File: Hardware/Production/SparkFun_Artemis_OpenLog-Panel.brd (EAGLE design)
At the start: 106.2 x 95.2 mm, 714 parts, among them J11 QWIIC_RIGHT_ANGLE, J14 CORTEX_JTAG, J16 CORTEX_JTAG, J17 MICRO-SD, J18 MICRO-SD, J19 QWIIC_RIGHT_ANGLE, J25 CORTEX_JTAG, J26 MICRO-SD, J27 QWIIC_RIGHT_ANGLE, J33 CORTEX_JTAG, J34 MICRO-SD, J35 QWIIC_RIGHT_ANGLE, J41 CORTEX_JTAG, J42 MICRO-SD, J43 QWIIC_RIGHT_ANGLE, J6 CORTEX_JTAG, J7 MICRO-SD, J8 QWIIC_RIGHT_ANGLE, Q1 20V/0.2A/8MHz/1.2Ω/1Vth, Q10 20V/0.2A/8MHz/1.2Ω/1Vth, Q11 20V/0.2A/8MHz/1.2Ω/1Vth, Q12 20V/4.2A/52mΩ/1.4W, Q13 20V/0.2A/8MHz/1.2Ω/1Vth, Q14 20V/0.2A/8MHz/1.2Ω/1Vth, Q15 20V/0.2A/8MHz/1.2Ω/1Vth, Q16 20V/0.2A/8MHz/1.2Ω/1Vth, Q17 20V/0.2A/8MHz/1.2Ω/1Vth, Q18 20V/4.2A/52mΩ/1.4W, Q19 20V/0.2A/8MHz/1.2Ω/1Vth, Q2 20V/0.2A/8MHz/1.2Ω/1Vth, Q20 20V/0.2A/8MHz/1.2Ω/1Vth, Q21 20V/0.2A/8MHz/1.2Ω/1Vth, Q22 20V/0.2A/8MHz/1.2Ω/1Vth, Q23 20V/0.2A/8MHz/1.2Ω/1Vth, Q24 20V/4.2A/52mΩ/1.4W, Q25 20V/0.2A/8MHz/1.2Ω/1Vth, Q26 20V/0.2A/8MHz/1.2Ω/1Vth, Q27 20V/0.2A/8MHz/1.2Ω/1Vth, Q28 20V/0.2A/8MHz/1.2Ω/1Vth, Q29 20V/0.2A/8MHz/1.2Ω/1Vth, Q3 20V/0.2A/8MHz/1.2Ω/1Vth, Q30 20V/4.2A/52mΩ/1.4W, Q31 20V/0.2A/8MHz/1.2Ω/1Vth, Q32 20V/0.2A/8MHz/1.2Ω/1Vth, Q33 20V/0.2A/8MHz/1.2Ω/1Vth, Q34 20V/0.2A/8MHz/1.2Ω/1Vth, Q35 20V/0.2A/8MHz/1.2Ω/1Vth, Q36 20V/4.2A/52mΩ/1.4W, Q4 20V/4.2A/52mΩ/1.4W, Q5 20V/0.2A/8MHz/1.2Ω/1Vth, Q6 20V/0.2A/8MHz/1.2Ω/1Vth, Q7 20V/0.2A/8MHz/1.2Ω/1Vth, Q8 20V/0.2A/8MHz/1.2Ω/1Vth, Q9 20V/0.2A/8MHz/1.2Ω/1Vth, U1 3.2V Supervisor, U10 CH340E, U11 AP2112K, U12 3.2V Supervisor, U13 ICM-20948, U14 1.8V/100mA, U15 MCP73831, U16 ARTEMIS_MODULESMD, U17 CH340E, U18 ICM-20948, U19 1.8V/100mA, U2 MCP73831, U20 AP2112K, U21 3.2V Supervisor, U22 MCP73831, U23 ARTEMIS_MODULESMD, U24 CH340E, U25 ICM-20948, U26 1.8V/100mA, U27 AP2112K, U28 3.2V Supervisor, U29 MCP73831, U3 AP2112K, U30 ARTEMIS_MODULESMD, U31 CH340E, U32 ICM-20948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

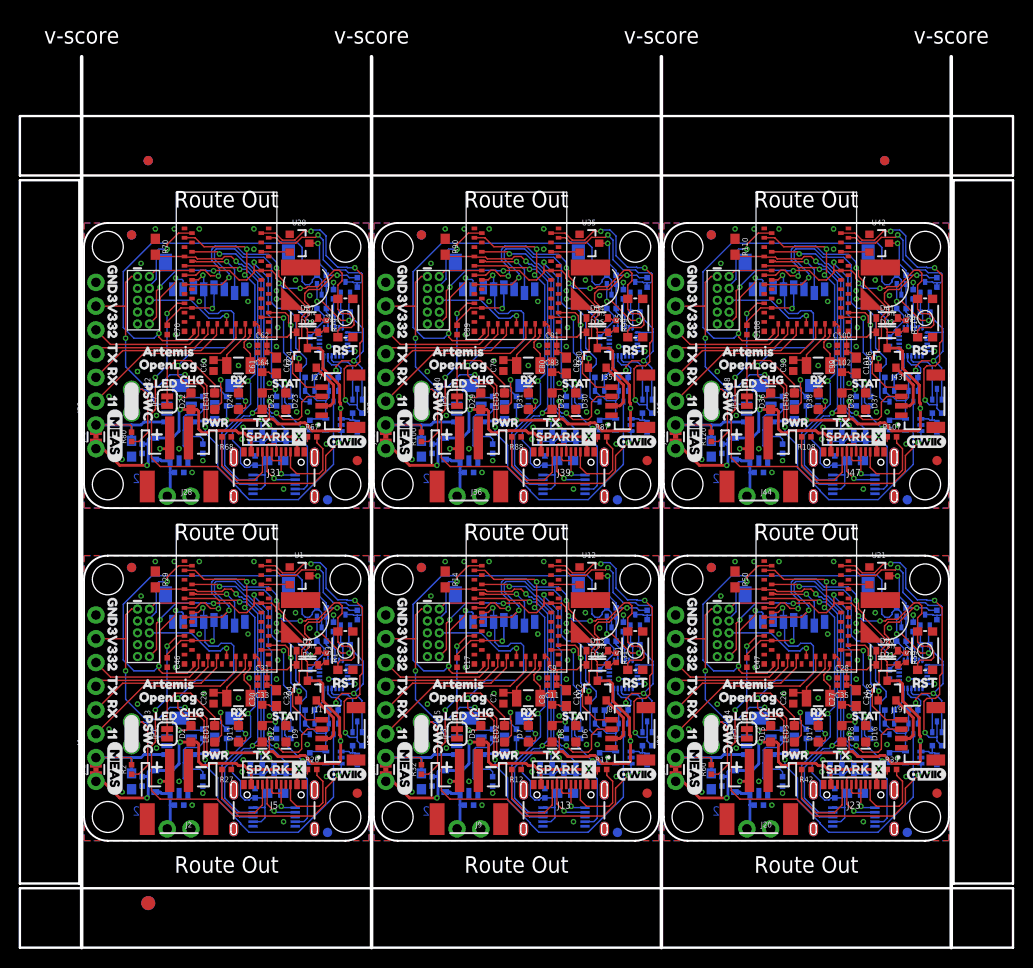
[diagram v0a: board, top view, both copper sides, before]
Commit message: PCB x03 commit for fab.
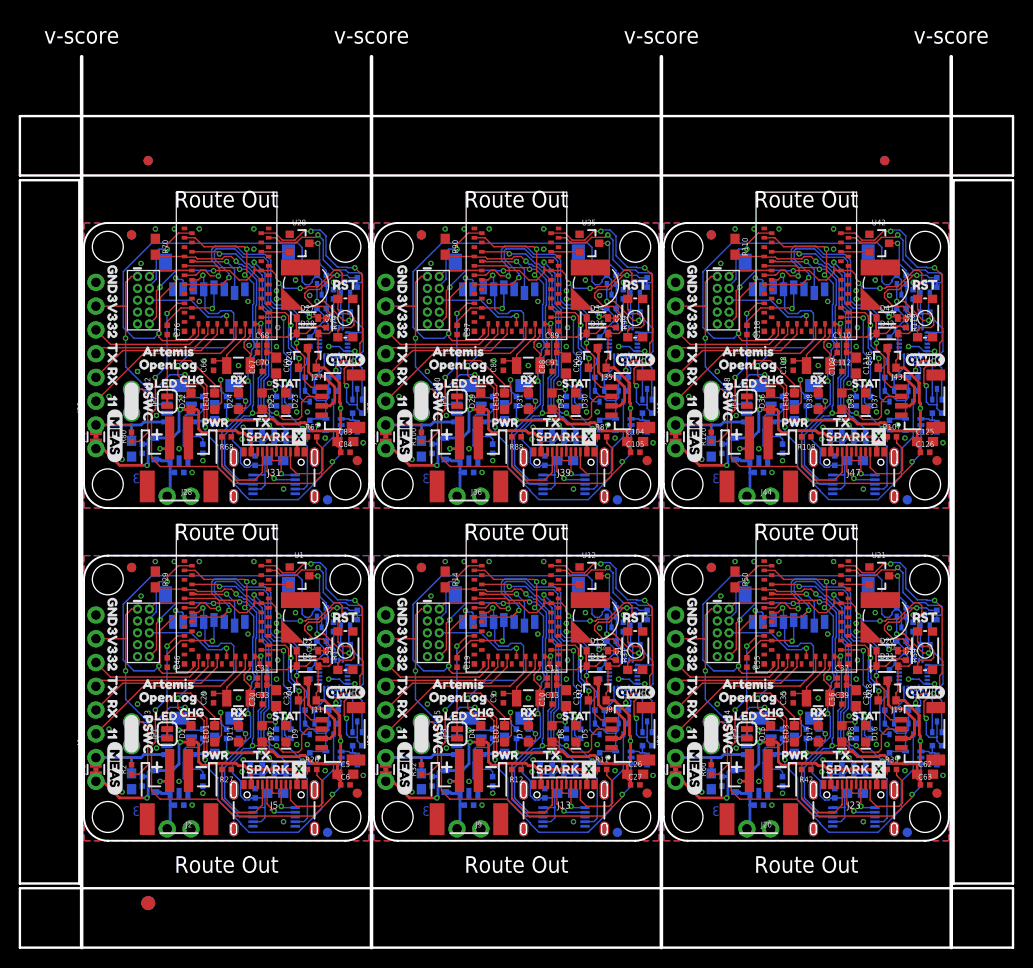
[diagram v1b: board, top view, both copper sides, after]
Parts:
- added C115, C116, C118, C119, C120: 0.1uF, SparkFun-Capacitors:0402-TIGHT
- added C117: 1.0nF, SparkFun-Capacitors:0402-TIGHT
- added C121, C122, C126: 1.0uF, SparkFun-Capacitors:0402-TIGHT
- added C123: 1.0uF, SparkFun-Capacitors:0603
- added C124: 2.2uF, SparkFun-Capacitors:0603
- added C125: 10uF, SparkFun-Capacitors:0603
- BT1, BT2, BT3, BT4, BT5, BT6: value ML414H_IV01E_BATTERY -> ML414H
- C10: value 10uF -> 15pF; device SparkFun-Capacitors:0603 -> SparkFun-Capacitors:0402-TIGHT
- C100, C105, C13, C39, C70, C91: value 0.1uF -> 1.0uF
- C101, C63: value 10uF -> 1.0uF; device SparkFun-Capacitors:0603 -> SparkFun-Capacitors:0402-TIGHT
- C102: device SparkFun-Capacitors:0402-TIGHT -> SparkFun-Capacitors:0603
- C103: value 10nF -> 2.2uF
- C104, C38, C62, C90: value 0.1uF -> 10uF; device SparkFun-Capacitors:0402-TIGHT -> SparkFun-Capacitors:0603
- C106, C28, C85, C86: value 0.1uF -> 4.7uF
- C107: value 1.0nF -> 4.7uF
- C108, C109, C66, C67, C87, C9: value 0.1uF -> 15pF
- C11, C20, C21, C55, C73, C74, C93: value 1.0uF -> 0.1uF
- C111, C83: value 1.0uF -> 10uF; device SparkFun-Capacitors:0402-TIGHT -> SparkFun-Capacitors:0603
- C113: value 1.0uF -> 10nF
- C114, C57, C76, C95: value 2.2uF -> 0.1uF; device SparkFun-Capacitors:0603 -> SparkFun-Capacitors:0402-TIGHT
- C12: value 10nF -> 10uF
- C14, C71: value 0.1uF -> 10nF; device SparkFun-Capacitors:0402-TIGHT -> SparkFun-Capacitors:0603
- C16: value 1.0nF -> 0.1uF
- C18: value 0.1uF -> 1.0nF
- C22: device SparkFun-Capacitors:0603 -> SparkFun-Capacitors:0402-TIGHT
- C23: value 2.2uF -> 1.0uF; device SparkFun-Capacitors:0603 -> SparkFun-Capacitors:0402-TIGHT
- C24: value 4.7uF -> 1.0uF; device SparkFun-Capacitors:0402-TIGHT -> SparkFun-Capacitors:0603
- C25: value 4.7uF -> 2.2uF; device SparkFun-Capacitors:0402-TIGHT -> SparkFun-Capacitors:0603
- C26: value 15pF -> 10uF; device SparkFun-Capacitors:0402 -> SparkFun-Capacitors:0603
- C27, C79, C80: value 15pF -> 1.0uF; device SparkFun-Capacitors:0402 -> SparkFun-Capacitors:0402-TIGHT
- C29, C30: device SparkFun-Capacitors:0402 -> SparkFun-Capacitors:0402-TIGHT
- C34: value 10uF -> 4.7uF; device SparkFun-Capacitors:0603 -> SparkFun-Capacitors:0402-TIGHT
- C35: value 1.0uF -> 15pF
- C36: value 10nF -> 15pF; device SparkFun-Capacitors:0603 -> SparkFun-Capacitors:0402-TIGHT
- C45: value 1.0nF -> 10nF; device SparkFun-Capacitors:0402-TIGHT -> SparkFun-Capacitors:0603
- C5: value 4.7uF -> 10uF; device SparkFun-Capacitors:0402-TIGHT -> SparkFun-Capacitors:0603
- C50: value 1.0uF -> 1.0nF
- C56, C94: value 1.0uF -> 0.1uF; device SparkFun-Capacitors:0603 -> SparkFun-Capacitors:0402-TIGHT
- C58, C59, C6: value 4.7uF -> 1.0uF
- C60: value 15pF -> 1.0uF; device SparkFun-Capacitors:0402 -> SparkFun-Capacitors:0603
- C61: value 15pF -> 2.2uF; device SparkFun-Capacitors:0402 -> SparkFun-Capacitors:0603
- C64: value 1.0uF -> 4.7uF
- C65: value 10nF -> 4.7uF; device SparkFun-Capacitors:0603 -> SparkFun-Capacitors:0402-TIGHT
- C69: value 1.0nF -> 10uF; device SparkFun-Capacitors:0402-TIGHT -> SparkFun-Capacitors:0603
- C7, C8: value 15pF -> 4.7uF; device SparkFun-Capacitors:0402 -> SparkFun-Capacitors:0402-TIGHT
- C75: value 1.0uF -> 1.0nF; device SparkFun-Capacitors:0603 -> SparkFun-Capacitors:0402-TIGHT
- C77, C78, C97: value 4.7uF -> 0.1uF
- C81: value 0.1uF -> 1.0uF; device SparkFun-Capacitors:0402-TIGHT -> SparkFun-Capacitors:0603
- C82: value 10uF -> 2.2uF
- C84: value 10nF -> 1.0uF; device SparkFun-Capacitors:0603 -> SparkFun-Capacitors:0402-TIGHT
- C88: value 1.0nF -> 15pF
- C92: value 1.0uF -> 10nF; device SparkFun-Capacitors:0402-TIGHT -> SparkFun-Capacitors:0603
- C96: value 4.7uF -> 1.0nF
- C98, C99: value 15pF -> 0.1uF; device SparkFun-Capacitors:0402 -> SparkFun-Capacitors:0402-TIGHT
- D14, D21, D28, D35, D42: value 3A/10V/280mV -> 1A/23V/620mV
- D4: value 3A/10V/280mV -> Yellow; device SparkFun-DiscreteSemi:SOD-323 -> SparkFun-LED:LED-0603
- D5: value Yellow -> BLUE
- D6: value BLUE -> 1A/23V/620mV; device SparkFun-LED:LED-0603 -> SparkFun-DiscreteSemi:SOD-323
- J11, J19, J27, J35, J43, J8: value QWIIC_RIGHT_ANGLE -> (none)
- moved C59 91.2 mm to (91.2, 8.64)
- moved C62 84.4 mm to (89.9, 7.11)
- moved C63 82.6 mm to (89.9, 5.97), turned to 0 degrees
- moved C58 79.0 mm to (86.1, 17.8), turned to 270 degrees
- moved C61 69.8 mm to (75.9, 10.2), flipped to the bottom
- moved C60 69.3 mm to (67.1, 6.35), flipped to the bottom, turned to 270 degrees
- moved C81 46.3 mm to (5.08, 41.9), flipped to the bottom, turned to 270 degrees
- moved C102 46.1 mm to (36.1, 41.9), flipped to the bottom, turned to 270 degrees
- moved C82 37.9 mm to (14.0, 45.7), flipped to the bottom, turned to 90 degrees
- moved C103 37.8 mm to (45.0, 45.7), turned to 90 degrees
- moved C24 36.2 mm to (36.1, 6.35), turned to 270 degrees
- moved C97 31.0 mm to (39.9, 54.6), flipped to the top
- moved D6 29.6 mm to (23.9, 18.7), turned to 0 degrees
- moved C56 27.2 mm to (88.6, 22.9), turned to 90 degrees
- moved C99 26.6 mm to (55.1, 44.5), flipped to the bottom, turned to 270 degrees
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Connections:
- net 3.3V: now also C5.1, C6.1, D6.A, Q4.2; no longer D4.A, Q4.3, R1.2, R28.2
- net 3.3V1: now also C14.1, C15.1, C25.1, C26.1, C27.1, Q12.2; no longer C12.1, C13.1, C21.1, Q12.3, R13.2, R31.2
- net 3.3V2: now also C45.1, C47.1, C59.1, C61.1, C62.1, C63.1, Q18.2; no longer C36.1, C37.1, C55.1, C57.1, Q18.3, R43.2, R59.2
- net 3.3V3: now also C71.1, C72.1, C80.1, C82.1, C83.1, C84.1, Q24.2; no longer C65.1, C66.1, C74.1, C76.1, Q24.3, R69.2, R79.2
- net 3.3V4: now also C101.1, C103.1, C104.1, C105.1, C92.1, Q30.2; no longer C84.1, C85.1, C95.1, Q30.3, R89.2, R99.2
- net 3.3V5: now also C113.1, C122.1, C124.1, C125.1, C126.1, Q36.2; no longer C103.1, C104.1, C112.1, Q36.3, R109.2, R119.2
- net 5V1: now also C8.1, D4.A; no longer C6.1, D5.A
- net 5V2: now also C34.1; no longer C25.1
- net 5V3: now also C65.1; no longer C59.1
- net 5V4: now also C86.1; no longer C78.1
- net 5V5: now also C107.1; no longer C97.1
- net ARTEMIS_!RESET1: now also C16.2, C18.1; no longer C14.2, C16.1
- net ARTEMIS_!RESET2: now also C48.2, C50.1; no longer C38.2, C45.1
- net ARTEMIS_!RESET3: now also C73.2, C75.1; no longer C67.2, C69.1
- net ARTEMIS_!RESET4: now also C94.2, C96.1; no longer C86.2, C88.1
- net ARTEMIS_!RESET5: now also C115.2, C117.1; no longer C105.2, C107.1
- net ARTEMIS_!RTS!1: now also C16.1, C17.1; no longer C14.1, C15.1
- net ARTEMIS_!RTS!2: now also C48.1, C49.1; no longer C38.1, C39.1
- net ARTEMIS_!RTS!3: now also C73.1, C74.1; no longer C67.1, C68.1
- net ARTEMIS_!RTS!4: now also C94.1, C95.1; no longer C86.1, C87.1
- net ARTEMIS_!RTS!5: now also C115.1, C116.1; no longer C105.1, C106.1
- net ARTEMIS_BOOT1: now also C17.2; no longer C15.2
- net ARTEMIS_BOOT2: now also C49.2; no longer C39.2
- net ARTEMIS_BOOT3: now also C74.2; no longer C68.2
- net ARTEMIS_BOOT4: now also C95.2; no longer C87.2
- net ARTEMIS_BOOT5: now also C116.2; no longer C106.2
- net GND: now also C5.2, C6.2
- net GND1: now also C10.1, C11.1, C14.2, C15.2, C24.2, C25.2, C26.2, C27.2, C7.2, C8.2, D5.C; no longer C10.2, C11.2, C16.2, C17.2, C5.2, C6.2, C7.1, C8.1, D6.C
- net GND2: now also C28.2, C35.1, C36.1, C37.1, C38.2, C39.2, C58.2, C59.2, C60.2, C61.2, C62.2, C63.2; no longer C24.2, C25.2, C26.1, C27.1, C28.1, C35.2, C36.2, C37.2, C48.2, C49.2
- net GND3: now also C66.1, C67.1, C68.1, C77.2, C78.2, C79.2, C80.2, C81.2, C82.2, C83.2, C84.2; no longer C58.2, C59.2, C60.1, C61.1, C62.1, C63.2, C66.2, C73.2, C74.2
- net GND4: now also C100.2, C101.2, C102.2, C103.2, C104.2, C105.2, C86.2, C87.1, C88.1, C89.1, C96.2, C97.2, C98.2, C99.2; no longer C77.2, C78.2, C79.1, C80.1, C81.1, C82.2, C83.2, C84.2, C88.2, C89.2, C94.2, C95.2
- net GND5: now also C106.2, C108.1, C109.1, C110.1, C117.2, C118.2, C119.2, C120.2, C121.2, C122.2, C123.2, C124.2, C125.2, C126.2; no longer C100.1, C101.2, C102.2, C103.2, C104.2, C108.2, C109.2, C110.2, C96.2, C97.2, C98.1, C99.1
- net ICM-20948-LV_#_1.8V1: now also C21.1, C22.1; no longer C19.1, C20.1
- net ICM-20948-LV_#_1.8V2: now also C57.1, C58.1; no longer C49.1, C50.1
- net ICM-20948-LV_#_1.8V3: now also C78.1, C79.1; no longer C72.1, C73.1
- net ICM-20948-LV_#_1.8V4: now also C100.1, C99.1; no longer C91.1, C92.1
- net ICM-20948-LV_#_1.8V5: now also C120.1, C121.1; no longer C110.1, C111.1
- net MICROSD_PWR1: now also C19.1; no longer C17.1
- net MICROSD_PWR2: now also C55.1; no longer C47.1
- net MICROSD_PWR3: now also C76.1; no longer C70.1
- net MICROSD_PWR4: now also C97.1; no longer C89.1
- net MICROSD_PWR5: now also C118.1; no longer C108.1
- net N$10: now also D5.A; no longer D6.A
- net N$14: now also C20.1; no longer C18.1
- net N$17: now also Q12.3; no longer Q12.2
- net N$22: now also C35.2; no longer C26.2
- net N$23: now also C36.2; no longer C27.2
- net N$3: now also D4.C; no longer D5.C
- net N$33: now also C56.1; no longer C48.1
- net N$36: now also Q18.3; no longer Q18.2
- net N$39: now also C66.2; no longer C60.2
- net N$40: now also C67.2; no longer C61.2
- net N$45: now also C77.1; no longer C71.1
- net N$48: now also Q24.3; no longer Q24.2
- net N$5: now also Q4.3; no longer Q4.2
- net N$51: now also C87.2; no longer C79.2
- net N$52: now also C88.2; no longer C80.2
- net N$57: now also C98.1; no longer C90.1
- net N$6: now also C9.2; no longer C7.2
- net N$60: now also Q30.3; no longer Q30.2
- net N$63: now also C108.2; no longer C98.2
- net N$64: now also C109.2; no longer C99.2
- net N$69: now also C119.1; no longer C109.1
- net N$72: now also Q36.3; no longer Q36.2
- net N$8: now also C10.2; no longer C8.2
- net VCC_1: now also D6.C, R1.2, R28.2; no longer D4.C
- net VCC_2: now also C11.2, C12.1, C13.1, R13.2, R31.2; no longer C10.1, C11.1, C9.2
- net VCC_3: now also C37.2, C38.1, C39.1, R43.2, R59.2; no longer C28.2, C34.1, C35.1
- net VCC_4: now also C68.2, C69.1, C70.1, R69.2, R79.2; no longer C62.2, C63.1, C64.1
- net VCC_5: now also C89.2, C90.1, C91.1, R89.2, R99.2; no longer C81.2, C82.1, C83.1
- net VCC_6: now also C110.2, C111.1, C112.1, R109.2, R119.2; no longer C100.2, C101.1, C102.1
- net VIN1: now also C24.1; no longer C22.1
- net VIN2: now also C60.1; no longer C56.1
- net VIN3: now also C81.1; no longer C75.1
- net VIN4: now also C102.1; no longer C94.1
- net VIN5: now also C123.1; no longer C113.1
- net V_BATT1: now also C7.1; no longer C5.1
- net V_BATT2: now also C28.1; no longer C24.1
- net V_BATT3: now also C64.1; no longer C58.1
- net V_BATT4: now also C85.1; no longer C77.1
- net V_BATT5: now also C106.1; no longer C96.1
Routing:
- net VCC_6: track 10.2 -> 26.6 mm, vias 0 -> 1
- net VCC_5: track 10.2 -> 26.6 mm, vias 0 -> 1
- net VCC_2: track 10.2 -> 26.6 mm, vias 0 -> 1
- net VCC_4: track 10.2 -> 26.6 mm, vias 0 -> 1
- net VCC_3: track 10.2 -> 26.6 mm, vias 0 -> 1
- net VCC_1: track 10.2 -> 26.6 mm, vias 0 -> 1
- net N$5: track 5.89 -> 9.18 mm
- net N$48: track 5.89 -> 9.18 mm
- net N$72: track 5.89 -> 9.18 mm
- net N$60: track 5.89 -> 9.18 mm
- net N$36: track 5.89 -> 9.18 mm
- net N$17: track 5.89 -> 9.18 mm
- net GND3: track 6.76 -> 5.17 mm
- net GND5: track 6.76 -> 5.17 mm
- net GND4: track 6.76 -> 5.17 mm
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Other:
- board text added: "x03"
- board text removed: "x02"
